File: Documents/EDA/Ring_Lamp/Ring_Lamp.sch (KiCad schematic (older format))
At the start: 20 parts, among them J101 Conn_01x02

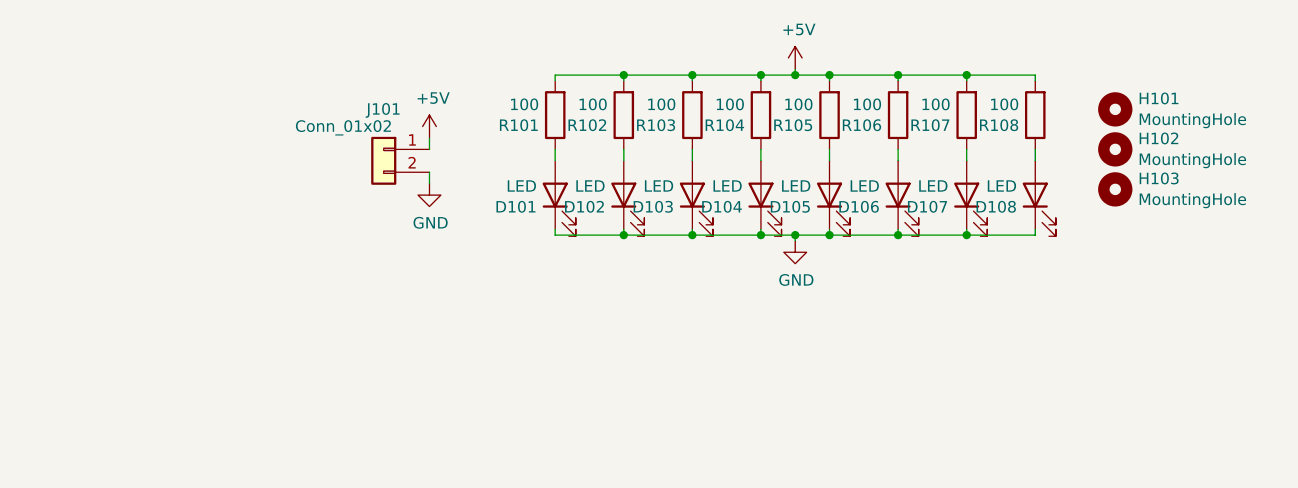
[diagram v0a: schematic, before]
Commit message: ring light
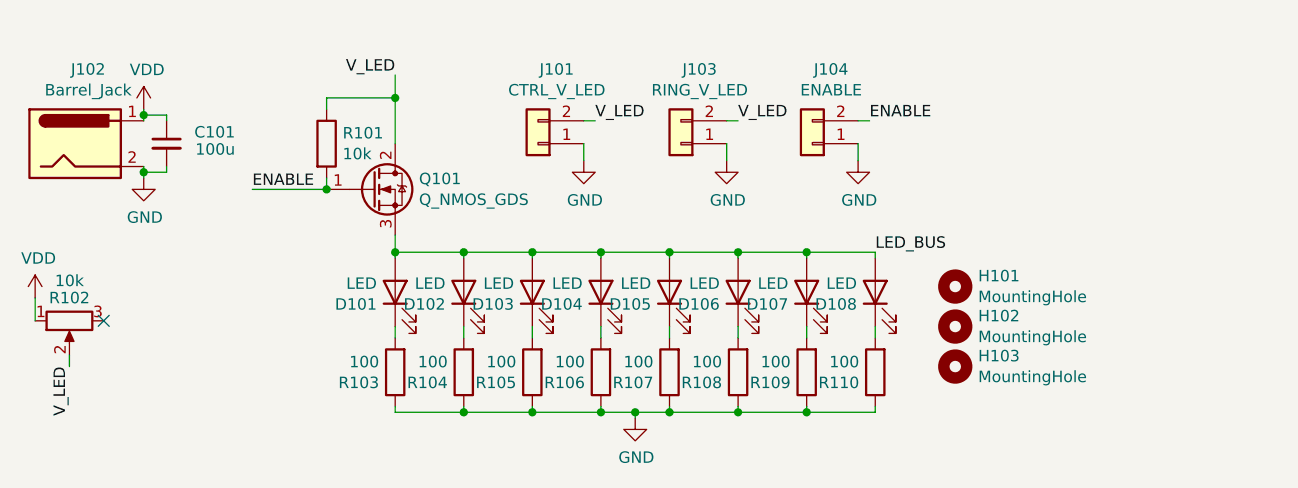
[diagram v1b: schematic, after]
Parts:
- removed R102: 100, Resistor_SMD:R_0805_2012Metric_Pad1.20x1.40mm_HandSolder, symbol Device:R
- added C101: 100u, Capacitor_THT:CP_Radial_D5.0mm_P2.50mm, symbol Device:C_Small
- added J102: Barrel_Jack, Connector_BarrelJack:BarrelJack_Horizontal, symbol Connector:Barrel_Jack
- added J103: RING_V_LED, TerminalBlock_Phoenix:TerminalBlock_Phoenix_MKDS-1,5-2_1x02_P5.00mm_Horizontal, symbol Connector_Generic:Conn_01x02
- added J104: ENABLE, Connector_PinHeader_2.54mm:PinHeader_1x02_P2.54mm_Vertical, symbol Connector_Generic:Conn_01x02
- added Q101: Q_NMOS_GDS, Package_TO_SOT_THT:TO-220-3_Vertical, symbol Device:Q_NMOS_GDS
- added R102: 10k, Potentiometer_THT:Potentiometer_Alps_RK09L_Single_Vertical, symbol Device:R_POT
- added R109, R110: 100, Resistor_SMD:R_0805_2012Metric_Pad1.20x1.40mm_HandSolder, symbol Device:R
- J101: value Conn_01x02 -> CTRL_V_LED; footprint footprints:USBA_Pads -> TerminalBlock_Phoenix:TerminalBlock_Phoenix_MKDS-1,5-2_1x02_P5.00mm_Horizontal
- R101: value 100 -> 10k
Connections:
- net GND: now also J101.1 (Pin_1), R103.1, R104.1, R105.1, R106.1, R107.1, R108.1, C101.2, J102.2, J103.1 (Pin_1), J104.1 (Pin_1), R109.1, R110.1; no longer D101.1 (K), D102.1 (K), D103.1 (K), D104.1 (K), D105.1 (K), D106.1 (K), D107.1 (K), D108.1 (K), J101.2 (Pin_2)
- net LED_BUS: now reaches D104.2 (A)
- net LED_BUS: now also D101.2 (A), D102.2 (A), D103.2 (A), D105.2 (A), D106.2 (A), D107.2 (A), D108.2 (A), Q101.3 (S); no longer R104.1
- net V_LED: now reaches R101.1
- net V_LED: now also J101.2 (Pin_2), J103.2 (Pin_2), Q101.2 (D), R102.2; no longer D101.2 (A)
- removed net +5V: J101.1 (Pin_1), R101.2, R103.2, R104.2, R105.2, R106.2, R107.2, R108.2
- new net: D104.1 (K), R106.2
- new net: D105.1 (K), R107.2
- new net: D103.1 (K), R105.2
- new net: D102.1 (K), R104.2
- new net: D101.1 (K), R103.2
- new net: D106.1 (K), R108.2
- new net: D107.1 (K), R109.2
- new net: D108.1 (K), R110.2
- new net ENABLE: J104.2 (Pin_2), Q101.1 (G), R101.2
- new net VDD: C101.1, J102.1, R102.1
- no-connect marks 0 -> 1
